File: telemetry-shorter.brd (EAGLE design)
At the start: 69.8 x 22.9 mm, 60 parts, among them SW1 B3U-1000P-2P-SMD, U1 ATSAMD21G18_QFN, U2 SPX3819M5-L-3-0, U3 MCP73831T-2ACI/OT, U4 MPU-9250, U5 SIM868, U6 BMP280, X1 JSTPH, X2 32.768, X3 ZX62-B-5PA, X4 104239-1430, X5 U-FL, X6 U-FL

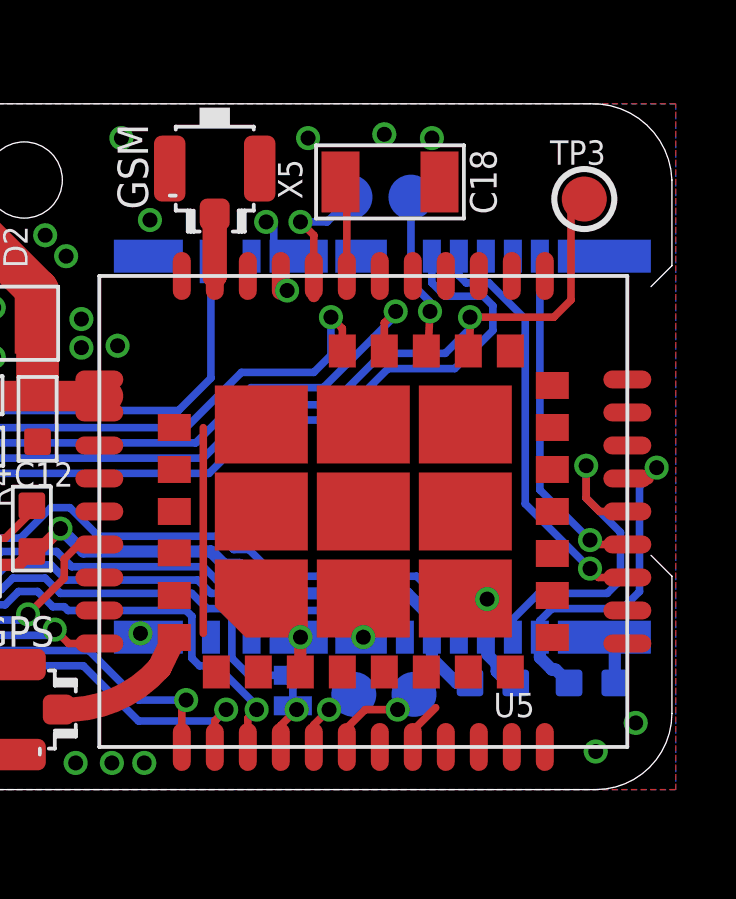
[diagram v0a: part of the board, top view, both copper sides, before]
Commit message: Small fixes
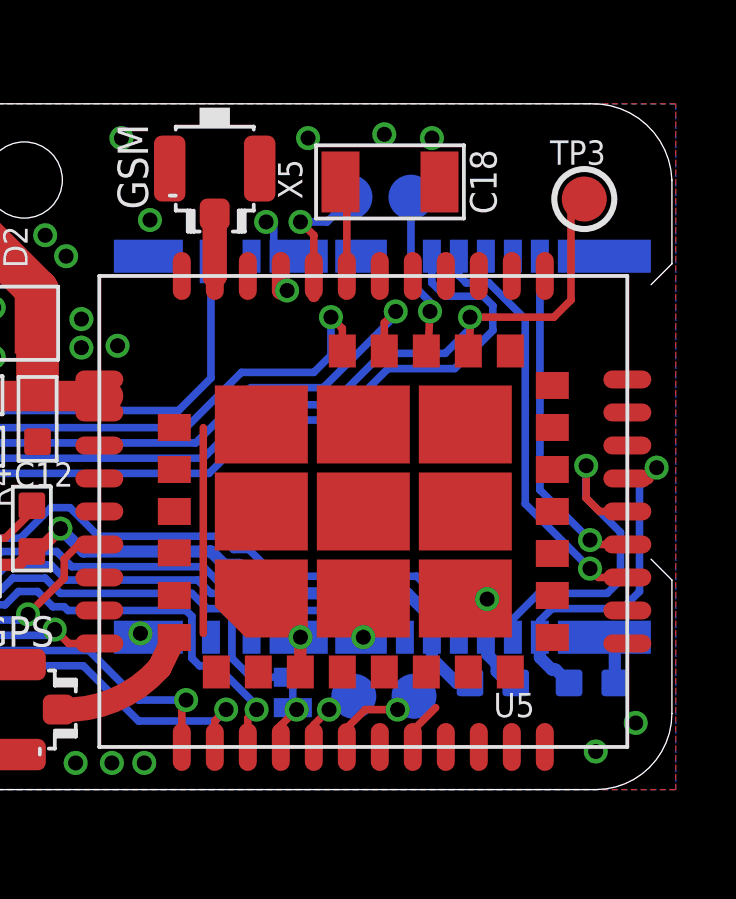
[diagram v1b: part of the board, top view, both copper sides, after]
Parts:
- moved JP2 0.06 mm to (57.2, 3.24)
- moved TP13 0.06 mm to (61.3, 3.11)
- moved TP6 0.06 mm to (59.2, 3.11)
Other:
- outline, holes or cut-outs redrawn
